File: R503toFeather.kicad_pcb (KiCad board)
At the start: 2 copper layers, 4 parts, among them J1 MX1.0 6P

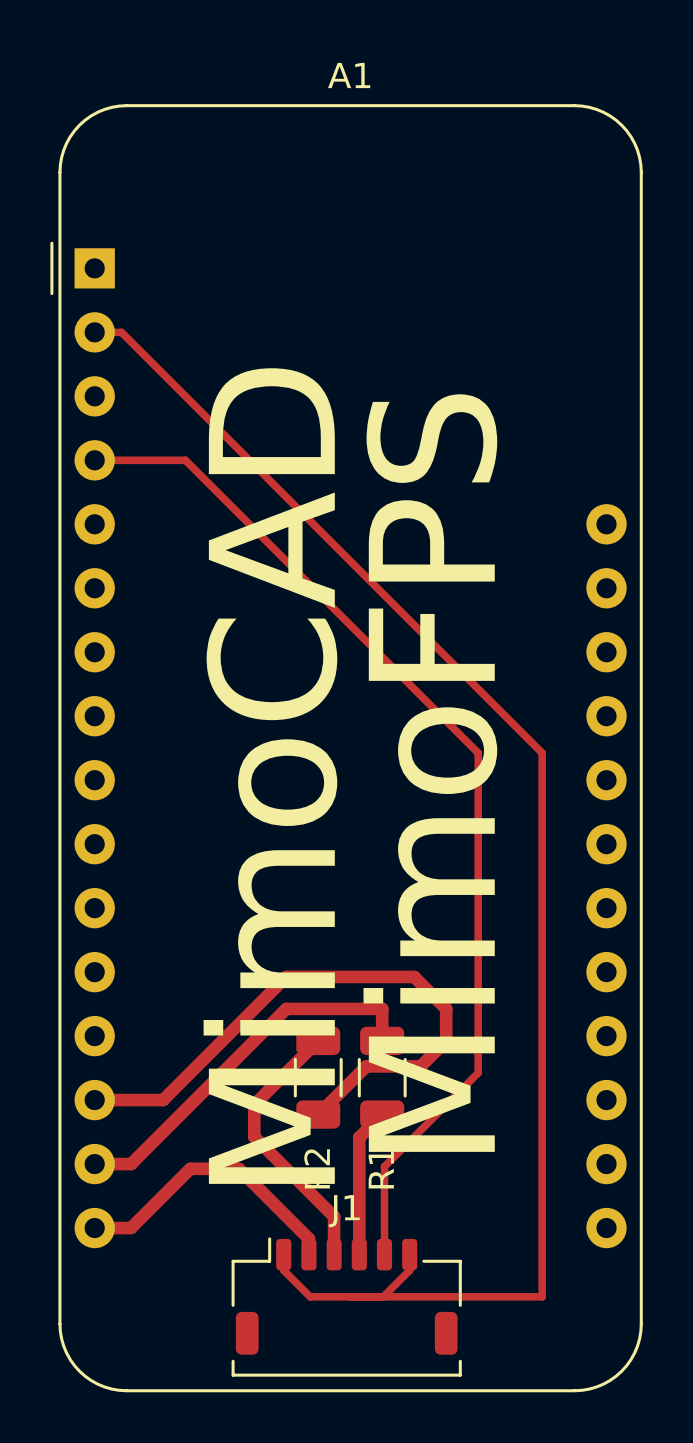
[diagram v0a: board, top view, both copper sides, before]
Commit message: RP2350 HSTX Production Version
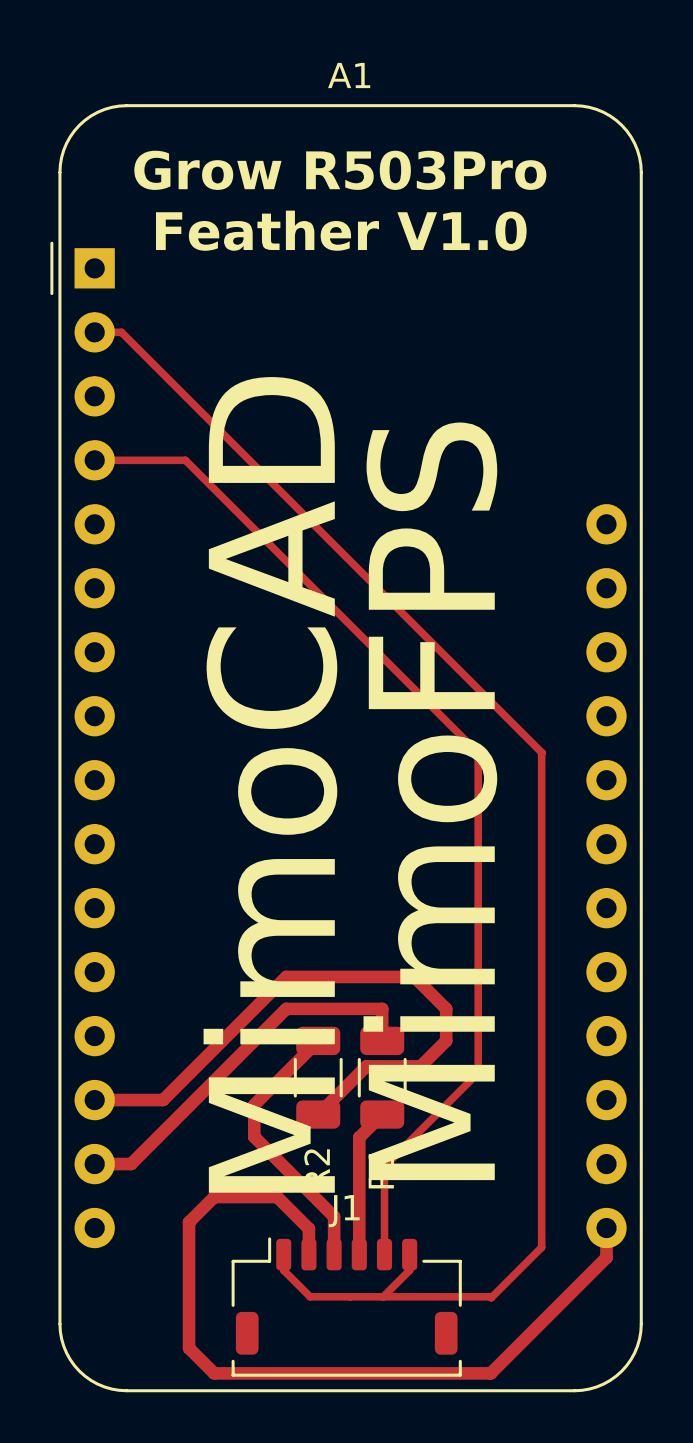
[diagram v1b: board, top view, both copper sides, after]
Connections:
- A1 pad 16: Net-(A1-SPARE) -> (no net)
- A1 pad 17: unconnected-(A1-SDA-Pad17) -> Net-(A1-SPARE)
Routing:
- net Net-(A1-SPARE): track 11.3 -> 31.8 mm
- net VCC: track 61.0 -> 58.6 mm
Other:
- board text added: "Grow R503Pro Feather V1.0"
